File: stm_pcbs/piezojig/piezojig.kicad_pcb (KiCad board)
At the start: 2 copper layers, 62.1 x 49 mm, 12 parts, among them P1 Z-XO, P10 SAMP, P11 GND, P12 SAMP, P13 GND, P2 Z-X, P4 Z-YO, P5 Z-Y, P6 Z+Y, P7 Z+YO, P8 Z+X, P9 Z+XO

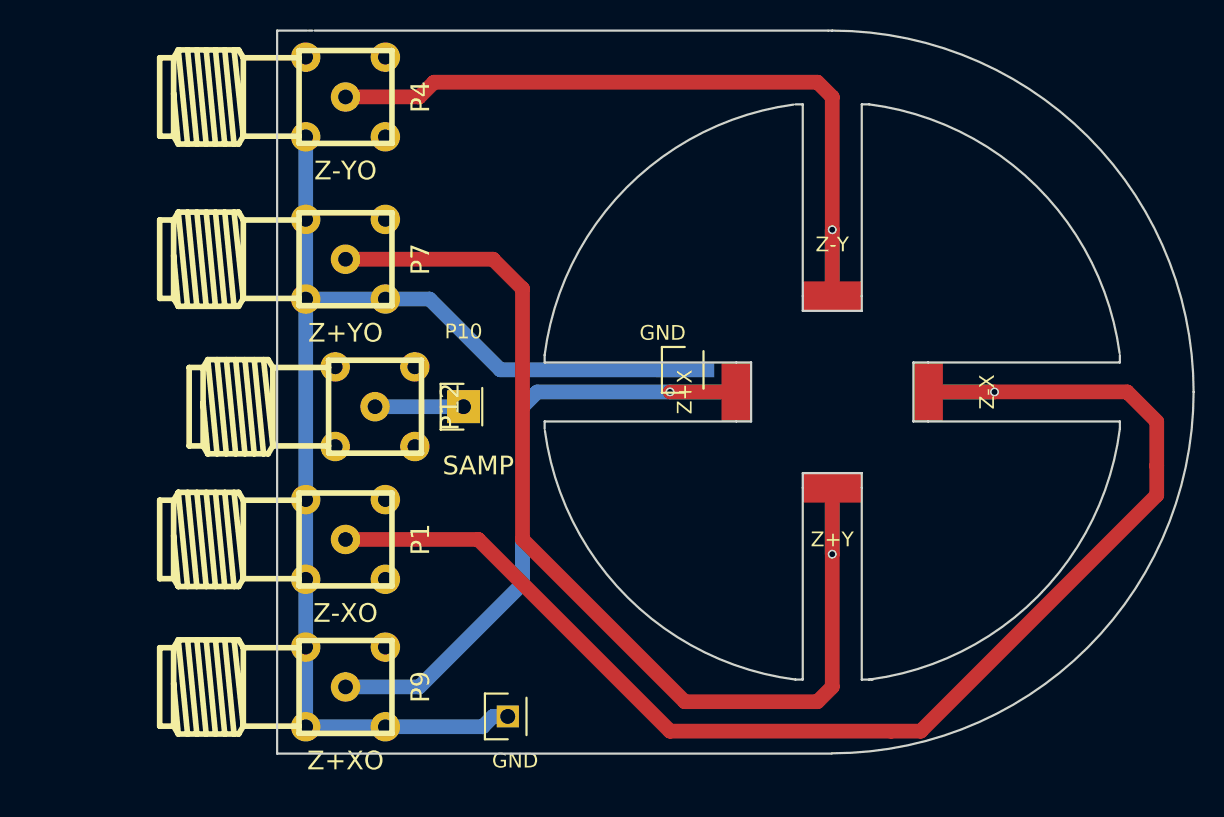
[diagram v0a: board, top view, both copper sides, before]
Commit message: misc
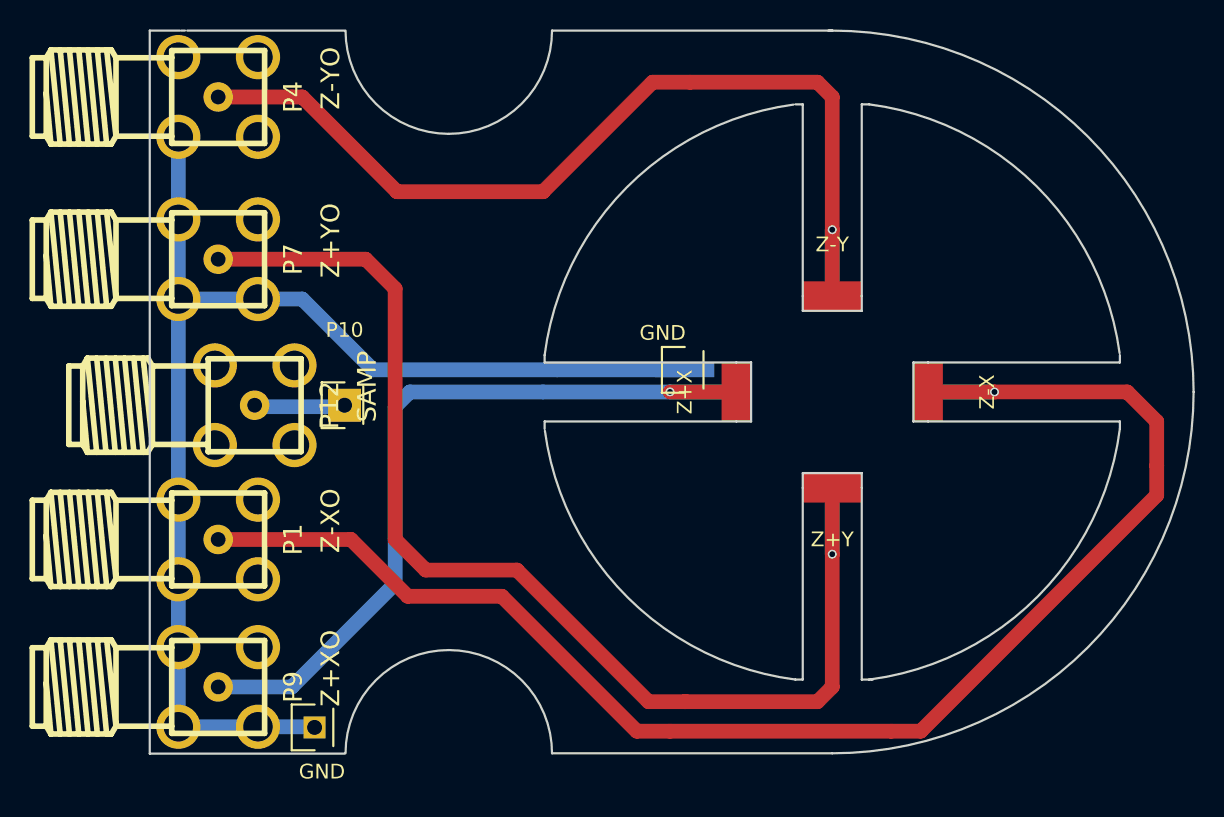
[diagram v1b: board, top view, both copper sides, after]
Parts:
- P1, P12, P4, P7, P9: footprint sma:SMA -> piezojig:SMA
- moved P11 13.1 mm to (104.9, 110.7)
- moved P1 8.64 mm to (98.4, 98.0)
- moved P4 8.64 mm to (98.4, 68.0)
- moved P7 8.64 mm to (98.4, 79.0)
- moved P9 8.64 mm to (98.4, 108.0)
- moved P12 8.16 mm to (100.8, 88.9)
- moved P10 8.07 mm to (106.9, 88.9)
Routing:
- net Net-(P4-Pad1): track 51.3 -> 65.3 mm
- net Net-(P6-Pad1): track 73.3 -> 82.0 mm
- net Net-(P8-Pad1): track 46.3 -> 54.9 mm
- net Net-(P1-Pad1): track 92.3 -> 101.0 mm
- net GND: track 81.7 -> 85.6 mm
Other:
- board size 62.1 x 49 mm -> 70.8 x 49 mm

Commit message: DDC112 board, multislope and various other updates it seems
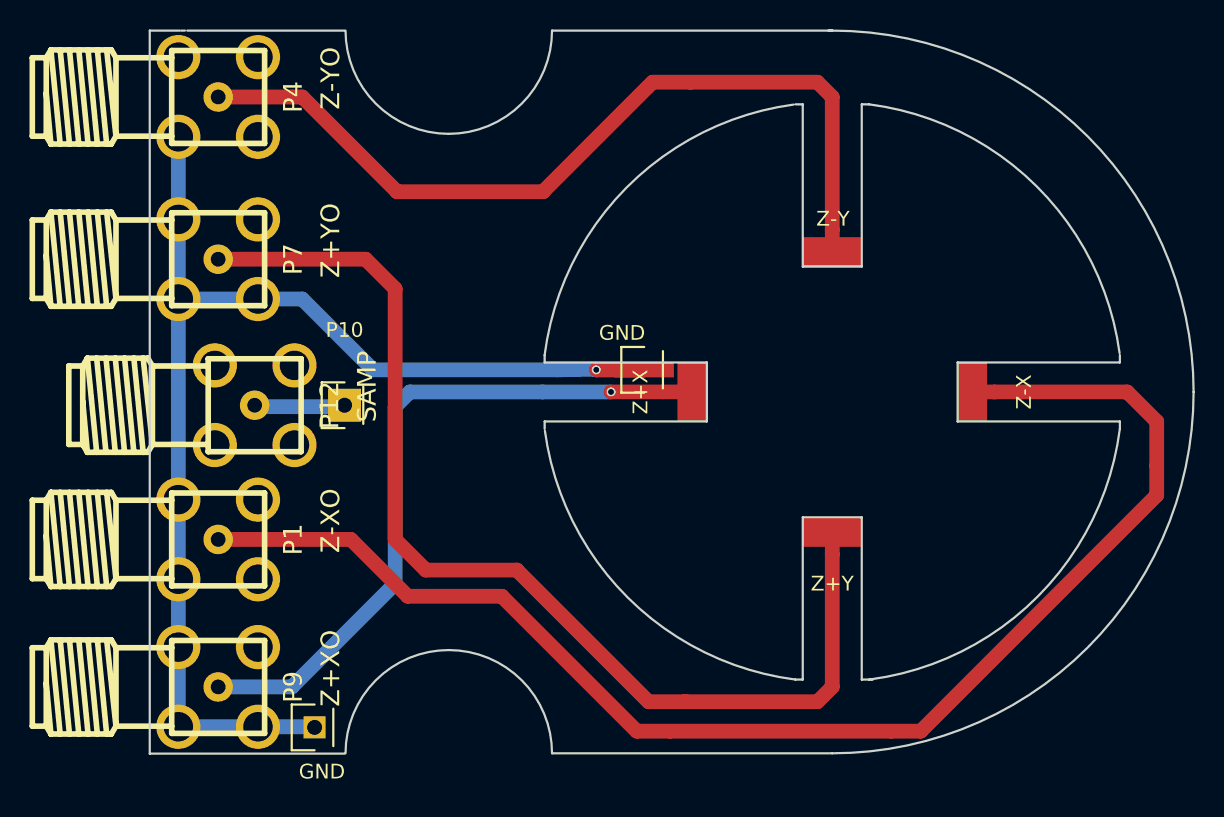
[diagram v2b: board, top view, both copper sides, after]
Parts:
- added P13: GND, Socket_Strips:Socket_Strip_Straight_1x01, B.Cu at (127.2, 86.5)
- P2, P5, P6, P8: footprint Socket_Strips:Socket_Strip_Straight_1x01 -> piezojig:piezopad
- moved P2 3.00 mm to (149.5, 88.0), turned to 180 degrees
- moved P5 3.00 mm to (140.0, 78.5)
- moved P6 3.00 mm to (140.0, 97.5)
- moved P8 3.00 mm to (130.5, 88.0)
- moved P13 2.75 mm to (127.2, 86.5)
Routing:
- net Net-(P8-Pad1): track 54.9 -> 47.8 mm
- net Net-(P1-Pad1): track 101.0 -> 94.2 mm, vias 1 -> 0
- net Net-(P6-Pad1): track 82.0 -> 75.2 mm, vias 1 -> 0
- net Net-(P4-Pad1): track 65.3 -> 58.5 mm, vias 1 -> 0
- net GND: track 85.6 -> 86.1 mm, vias 0 -> 1
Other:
- outline, holes or cut-outs redrawn
